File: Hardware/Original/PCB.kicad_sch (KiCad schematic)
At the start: 13 parts, among them J2 Conn_01x06, SW1 TS04-66-43-BK-100-SMT, U1 ME54BS01_V1.0, U3 MCP1700x-330xxTT

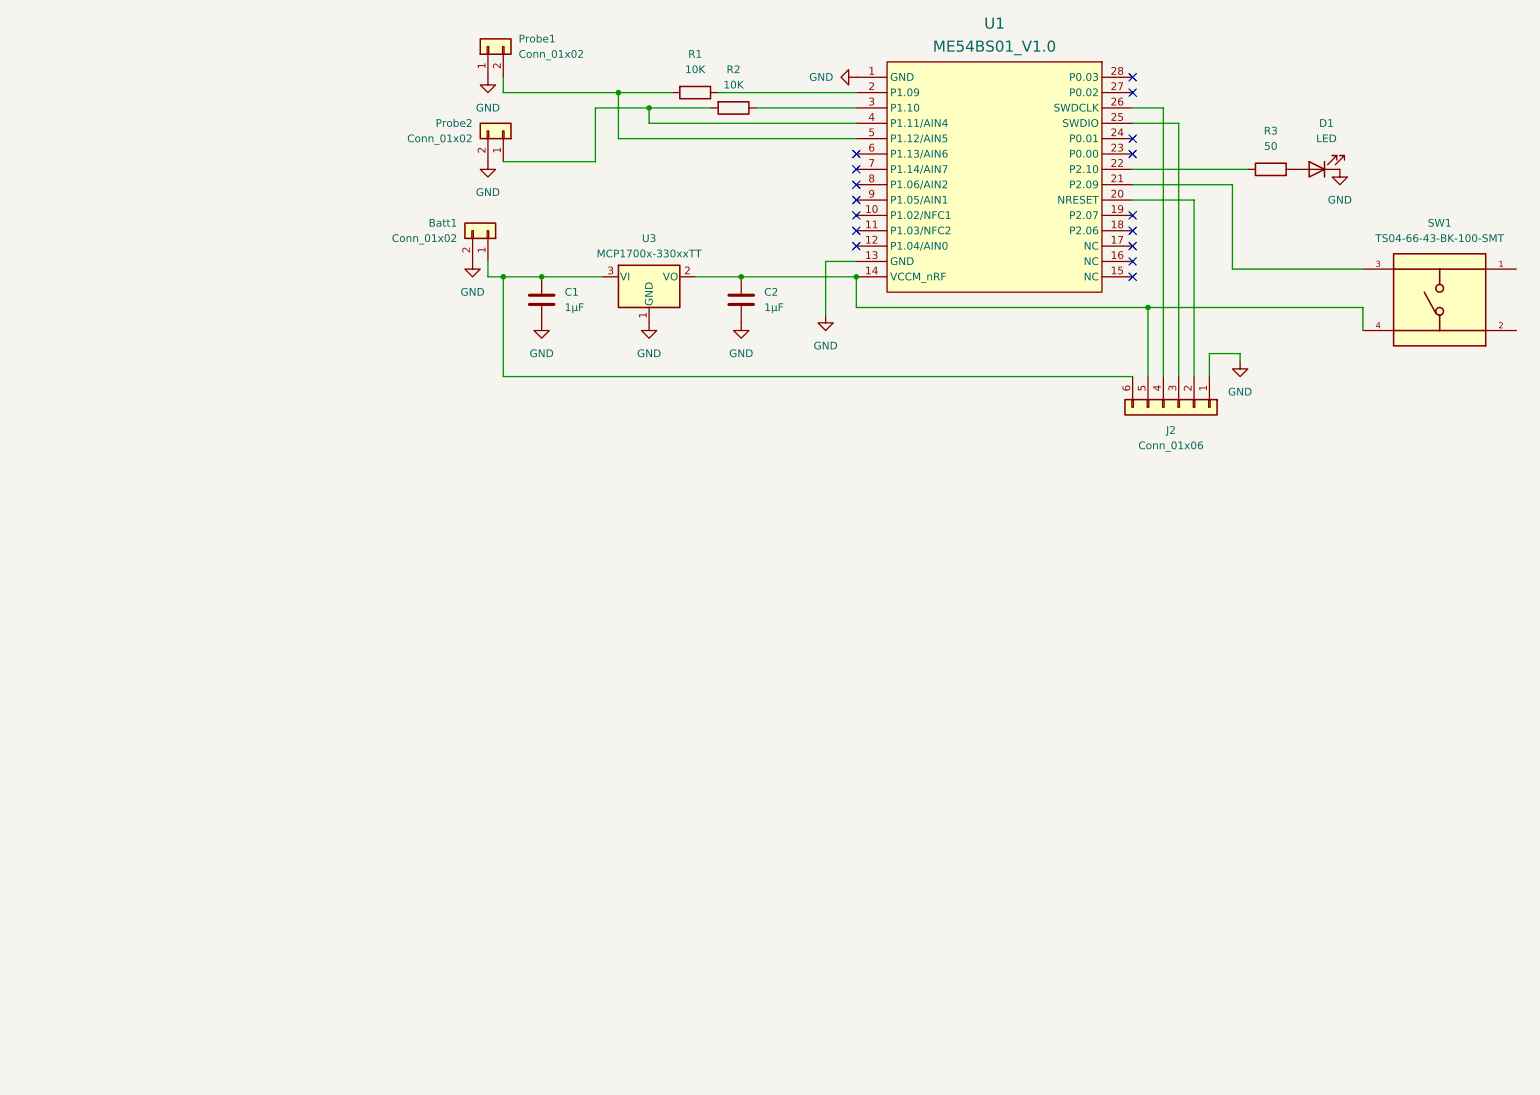
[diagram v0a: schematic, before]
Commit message: WIP
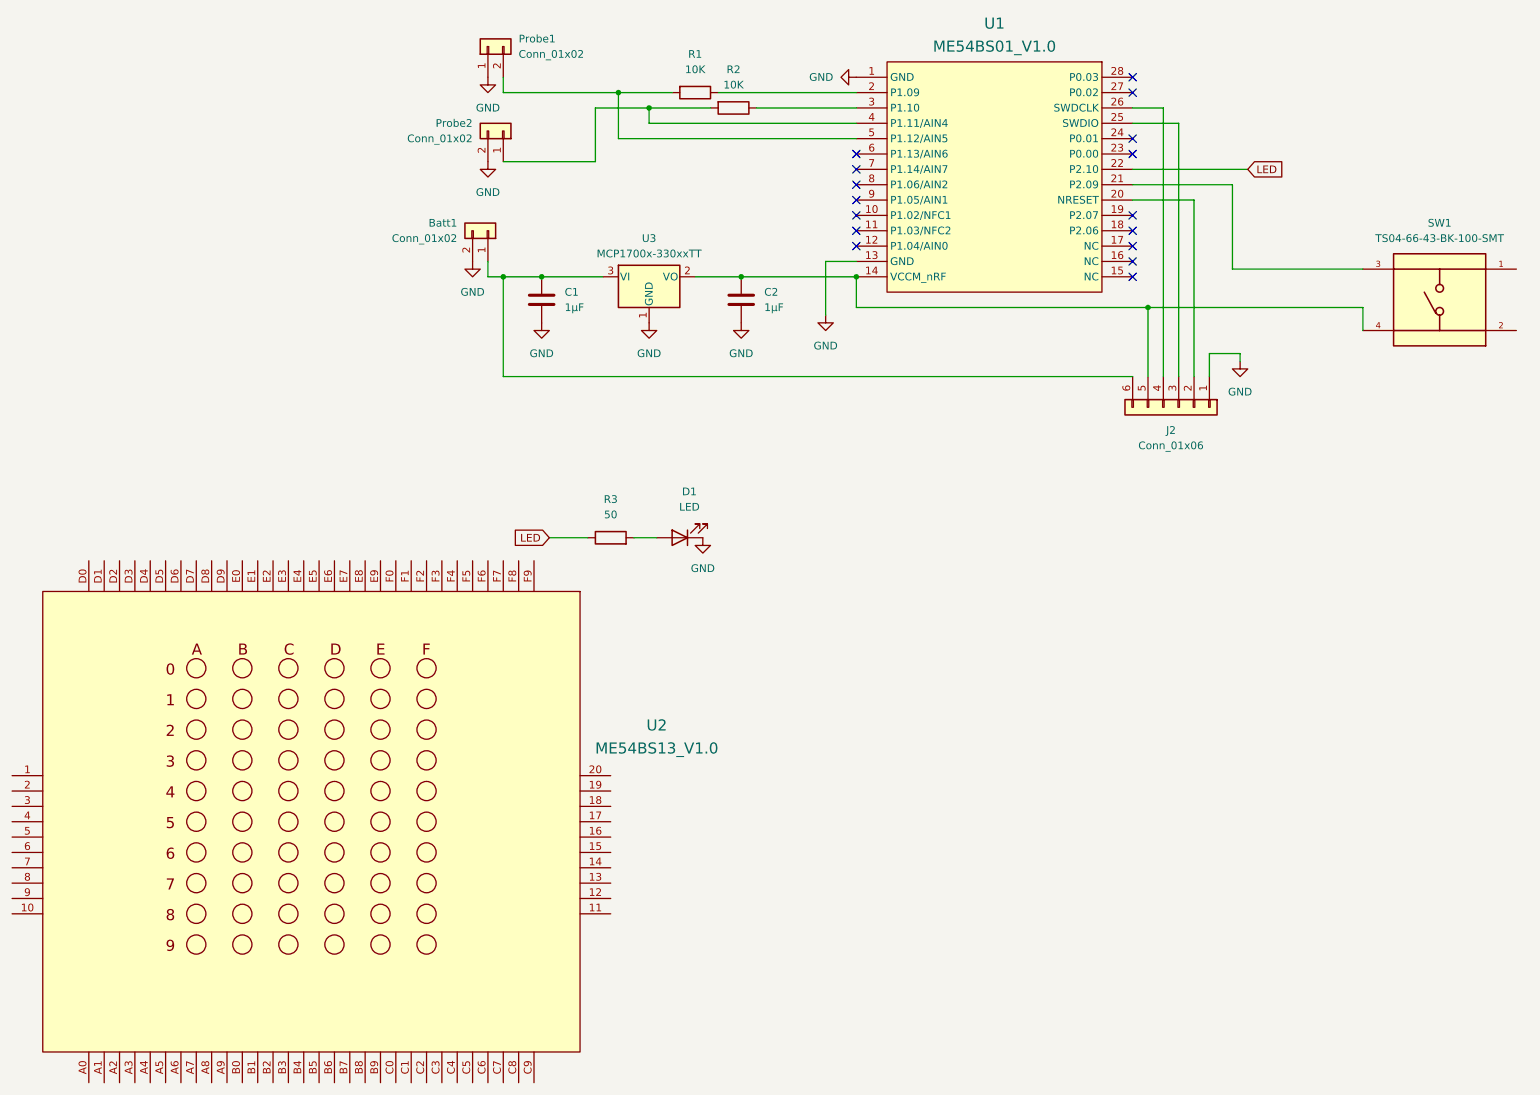
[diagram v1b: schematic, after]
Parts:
- added U2: ME54BS13_V1.0, ME54BS13_V1.0, symbol MS54B13:ME54BS13_V1.0
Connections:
- net LED: now reaches R3.1, U1.22 (P2.10)
